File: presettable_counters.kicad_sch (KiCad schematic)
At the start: 13 parts, among them J1 Conn_01x13, J2 Conn_02x05_Odd_Even, J3 Conn_02x12_Odd_Even, J4 Conn_01x13, U1 74HC191, U2 74HC191, U3 74HC191, U4 74HC245, U5 74HC245

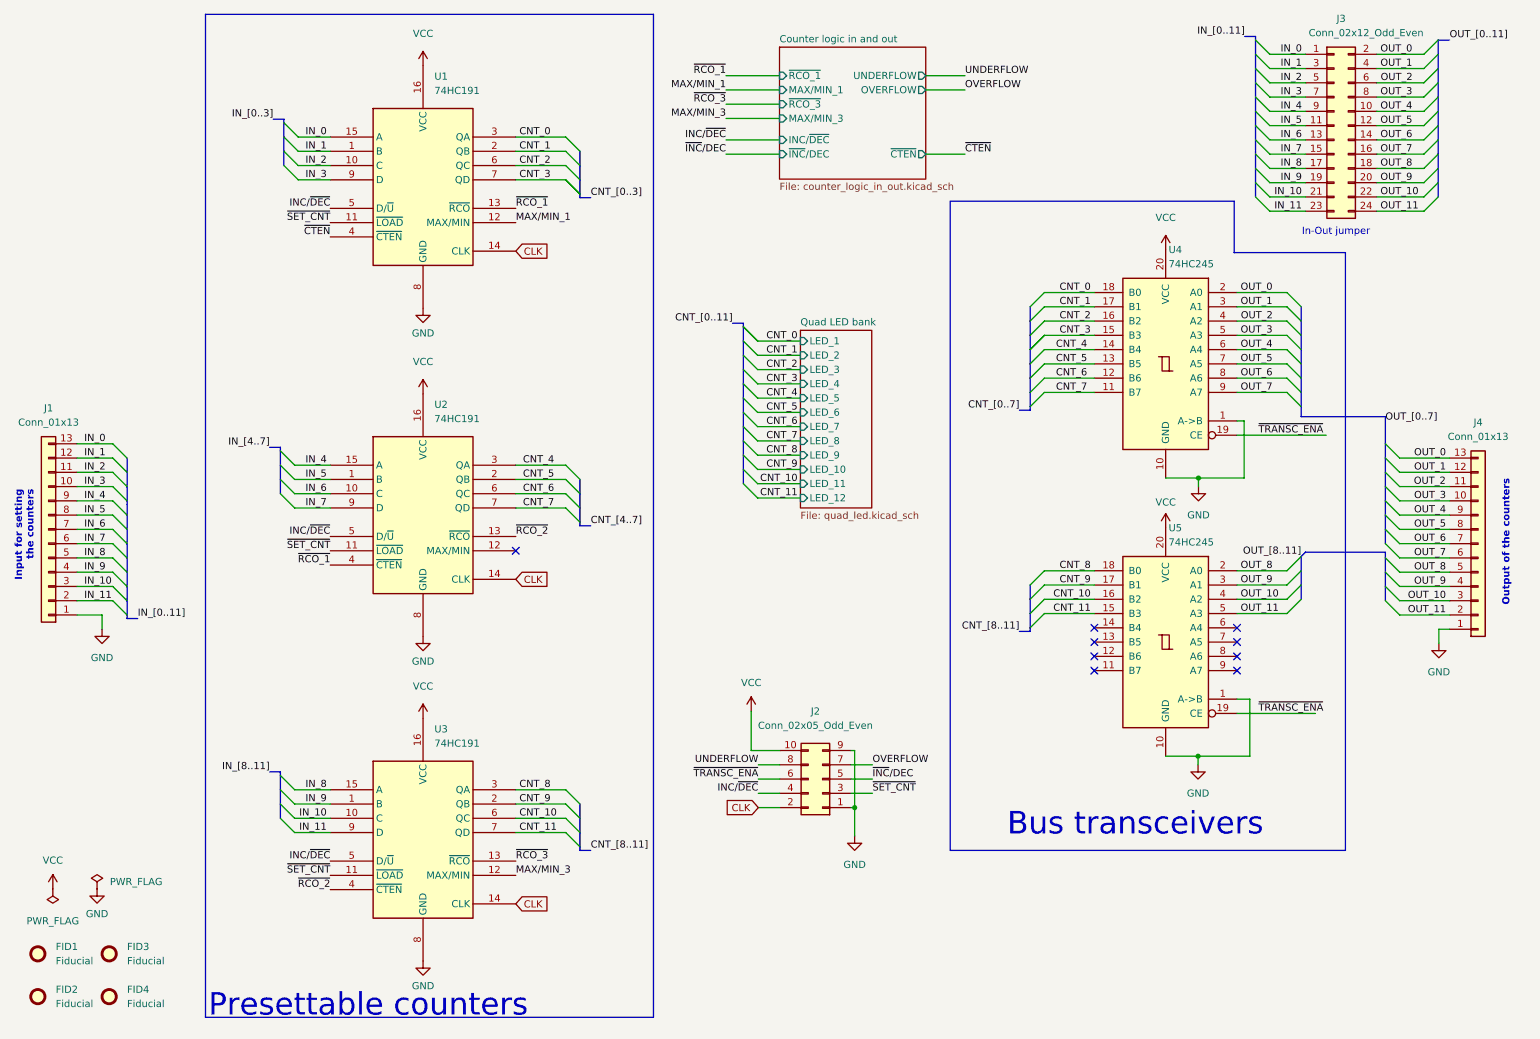
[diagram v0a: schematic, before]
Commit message: Trace the layout
- Place components on PCB
- Add silkscreeen
- Add traces
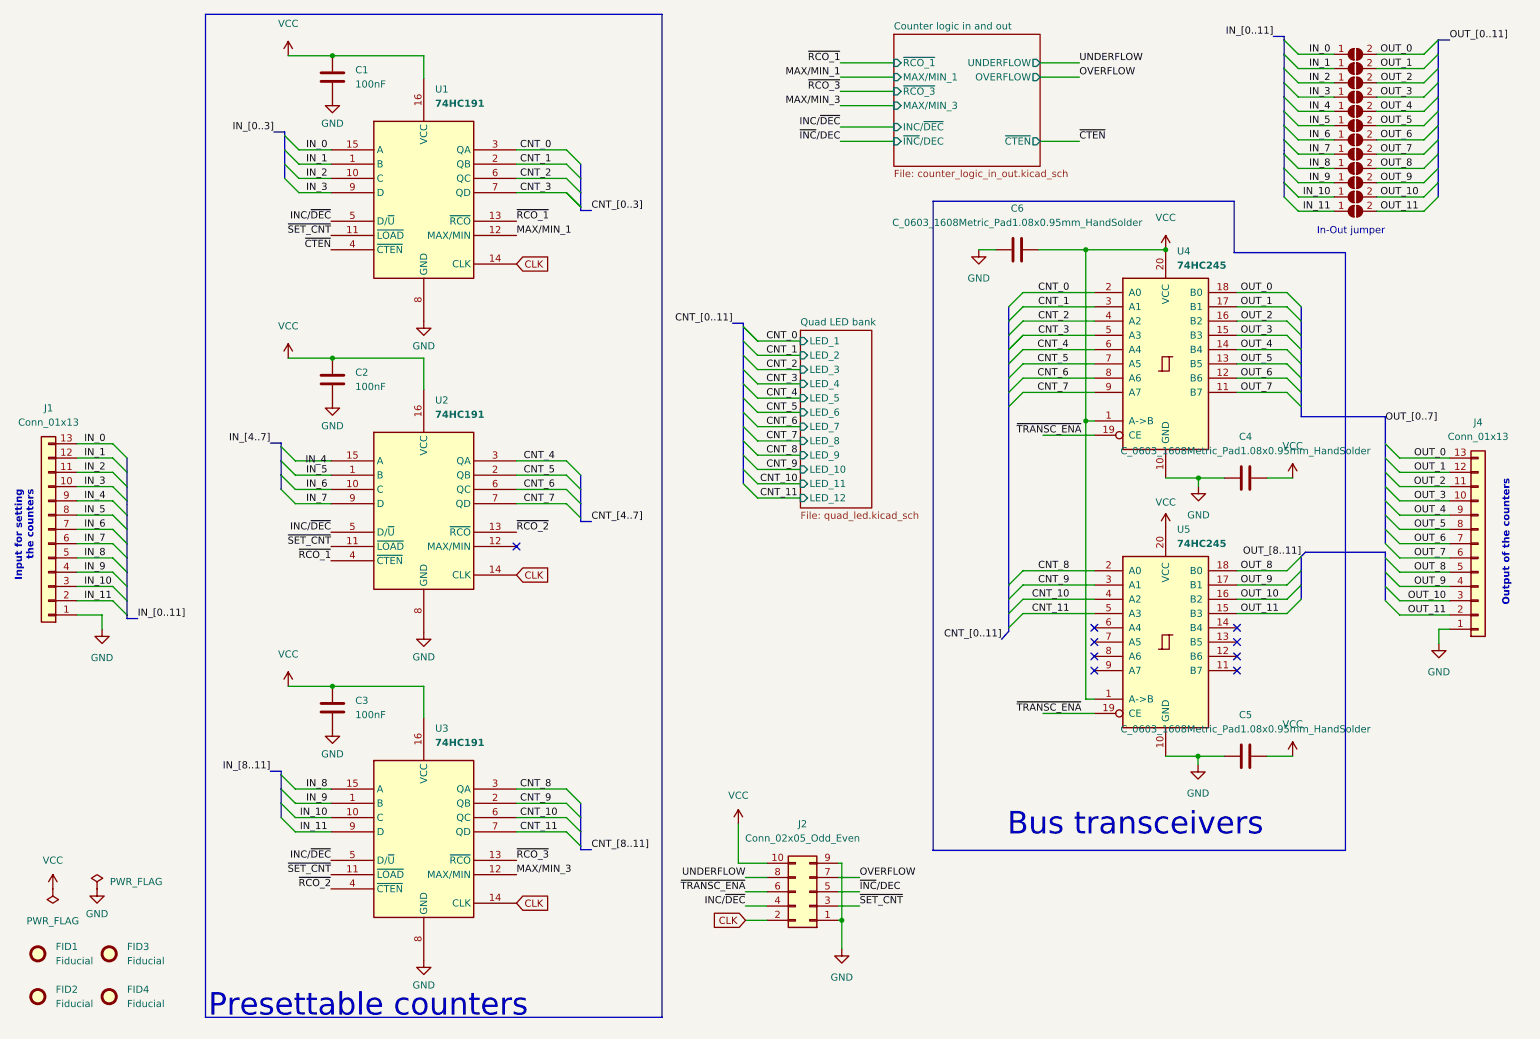
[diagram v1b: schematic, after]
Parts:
- added C1, C2, C3: 100nF, symbol Device:C
- added C4, C5, C6: C_0603_1608Metric_Pad1.08x0.95mm_HandSolder, Capacitor_SMD:C_0603_1608Metric_Pad1.08x0.95mm_HandSolder, symbol Device:C
- added J10, J11, J12, J13, J14, J15, J5, J6, J7, J8, J9: Conn_02x12_Odd_Even, Jumper:SolderJumper-2_P1.3mm_Open_RoundedPad1.0x1.5mm, symbol Jumper:SolderJumper_2_Open
- FID1, FID2, FID3, FID4: footprint (none) -> Fiducial:Fiducial_1.5mm_Mask3mm
- J3: footprint Connector_PinHeader_2.54mm:PinHeader_2x12_P2.54mm_Vertical -> Jumper:SolderJumper-2_P1.3mm_Open_RoundedPad1.0x1.5mm; symbol Connector_Generic:Conn_02x12_Odd_Even -> Jumper:SolderJumper_2_Open
- U4, U5: footprint footprints:TSSOP20B-M -> Package_SO:SOIC-20W_7.5x12.8mm_P1.27mm
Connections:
- net CNT_0: now also U4.2 (A0); no longer U4.18 (B0)
- net CNT_1: now also U4.3 (A1); no longer U4.17 (B1)
- net CNT_10: now also U5.4 (A2); no longer U5.16 (B2)
- net CNT_11: now also U5.5 (A3); no longer U5.15 (B3)
- net CNT_2: now also U4.4 (A2); no longer U4.16 (B2)
- net CNT_3: now also U4.5 (A3); no longer U4.15 (B3)
- net CNT_4: now also U4.6 (A4); no longer U4.14 (B4)
- net CNT_5: now also U4.7 (A5); no longer U4.13 (B5)
- net CNT_6: now also U4.8 (A6); no longer U4.12 (B6)
- net CNT_7: now also U4.9 (A7); no longer U4.11 (B7)
- net CNT_8: now also U5.2 (A0); no longer U5.18 (B0)
- net CNT_9: now also U5.3 (A1); no longer U5.17 (B1)
- net GND: now also C1.2, C2.2, C3.2, C4.1, C5.1, C6.1; no longer U4.1 (A->B), U5.1 (A->B)
- net IN_1: now also J5.1 (A); no longer J3.3 (Pin_3)
- net IN_10: now also J14.1 (A); no longer J3.21 (Pin_21)
- net IN_11: now also J15.1 (A); no longer J3.23 (Pin_23)
- net IN_2: now also J6.1 (A); no longer J3.5 (Pin_5)
- net IN_3: now also J7.1 (A); no longer J3.7 (Pin_7)
- net IN_4: now also J8.1 (A); no longer J3.9 (Pin_9), U2.15 (A)
- net IN_5: now also J9.1 (A); no longer J3.11 (Pin_11)
- net IN_6: now also J10.1 (A); no longer J3.13 (Pin_13)
- net IN_7: now also J11.1 (A); no longer J3.15 (Pin_15)
- net IN_8: now also J12.1 (A); no longer J3.17 (Pin_17)
- net IN_9: now also J13.1 (A); no longer J3.19 (Pin_19)
- net OUT_0: now also U4.18 (B0); no longer U4.2 (A0)
- net OUT_1: now also U4.17 (B1), J5.2 (B); no longer J3.4 (Pin_4), U4.3 (A1)
- net OUT_10: now also U5.16 (B2), J14.2 (B); no longer J3.22 (Pin_22), U5.4 (A2)
- net OUT_11: now also U5.15 (B3), J15.2 (B); no longer J3.24 (Pin_24), U5.5 (A3)
- net OUT_2: now also U4.16 (B2), J6.2 (B); no longer J3.6 (Pin_6), U4.4 (A2)
- net OUT_3: now also U4.15 (B3), J7.2 (B); no longer J3.8 (Pin_8), U4.5 (A3)
- net OUT_4: now also U4.14 (B4), J8.2 (B); no longer J3.10 (Pin_10), U4.6 (A4)
- net OUT_5: now also U4.13 (B5), J9.2 (B); no longer J3.12 (Pin_12), U4.7 (A5)
- net OUT_6: now also U4.12 (B6), J10.2 (B); no longer J3.14 (Pin_14), U4.8 (A6)
- net OUT_7: now also U4.11 (B7), J11.2 (B); no longer J3.16 (Pin_16), U4.9 (A7)
- net OUT_8: now also U5.18 (B0), J12.2 (B); no longer J3.18 (Pin_18), U5.2 (A0)
- net OUT_9: now also U5.17 (B1), J13.2 (B); no longer J3.20 (Pin_20), U5.3 (A1)
- net VCC: now also U4.1 (A->B), U5.1 (A->B), C1.1, C2.1, C3.1, C4.2, C5.2, C6.2
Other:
- moved on the sheet: J2, U1, U2
